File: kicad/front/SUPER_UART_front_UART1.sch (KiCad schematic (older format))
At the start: 67 parts, among them CON4 UART A, CON5 UART A, CON6 UART D, Q2 PDTA143ZT, Q3 2N7002PS, Q4 PDTA143ZT, Q5 2N7002PS, Q6 N-MOS_small, U10 LP2951CD, U7 74LVC8T245PW, U8 74LVC8T245PW, U9 74LVC1T45GW

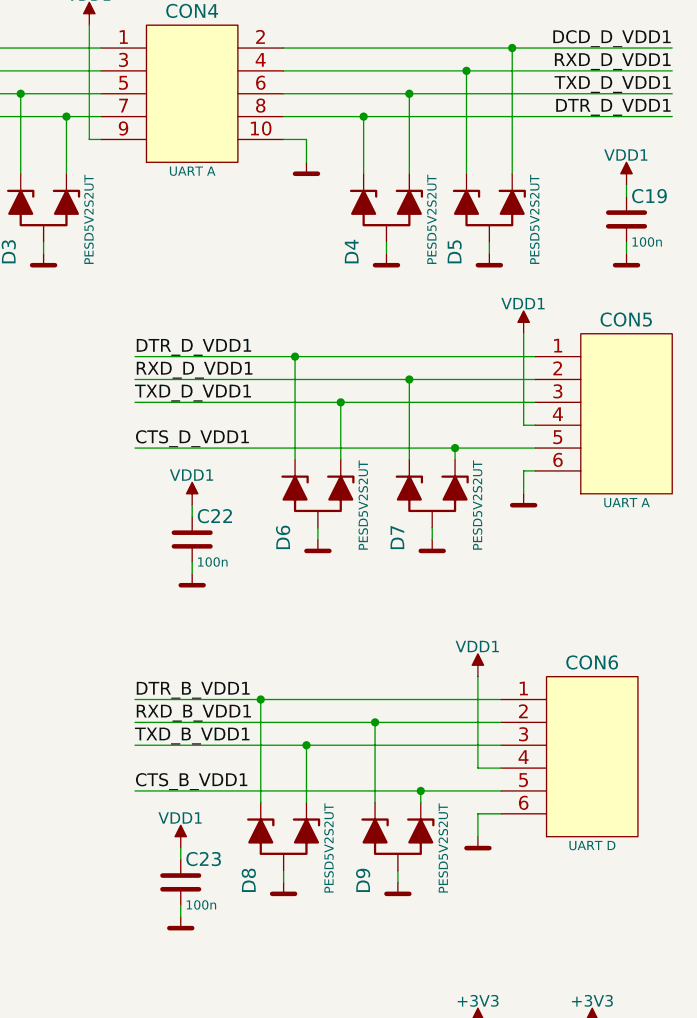
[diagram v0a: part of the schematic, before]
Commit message: Working on schematic
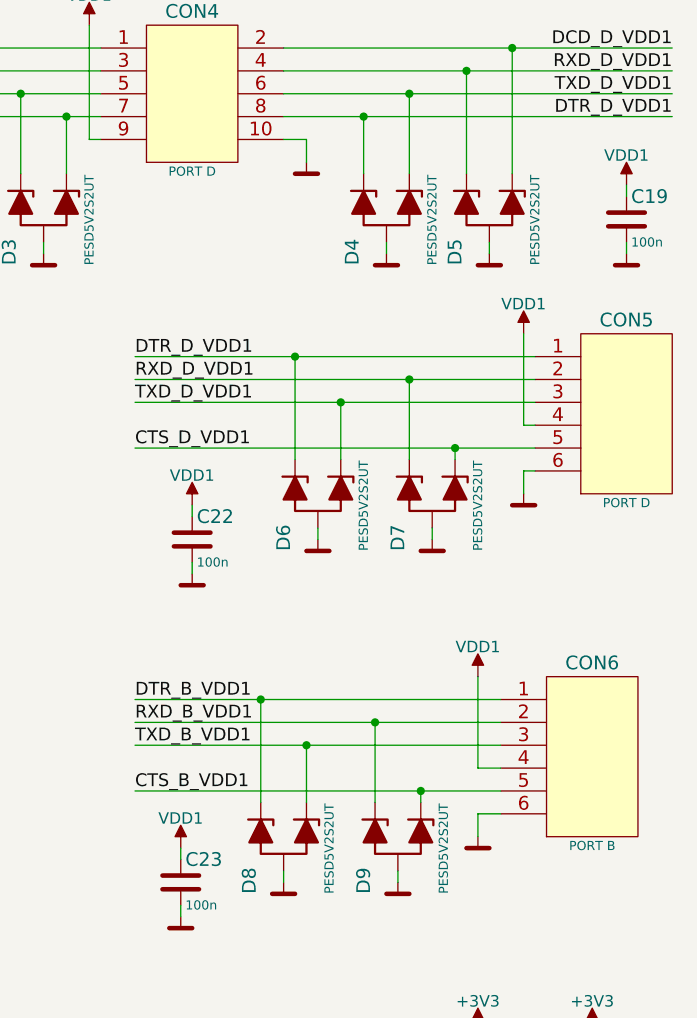
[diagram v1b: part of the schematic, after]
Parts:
- CON4, CON5: value UART A -> PORT D
- CON6: value UART D -> PORT B
- LED27, LED28, LED29, LED30, LED31, LED32, LED33, LED34: footprint pnSemiconductor:LED0603_R -> pnSemiconductor:0805D
